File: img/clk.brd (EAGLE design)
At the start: 59.4 x 51.4 mm, 27 parts, among them IC1 MEGA8-P, IC2 DS1307, J1 22-27-2021-02

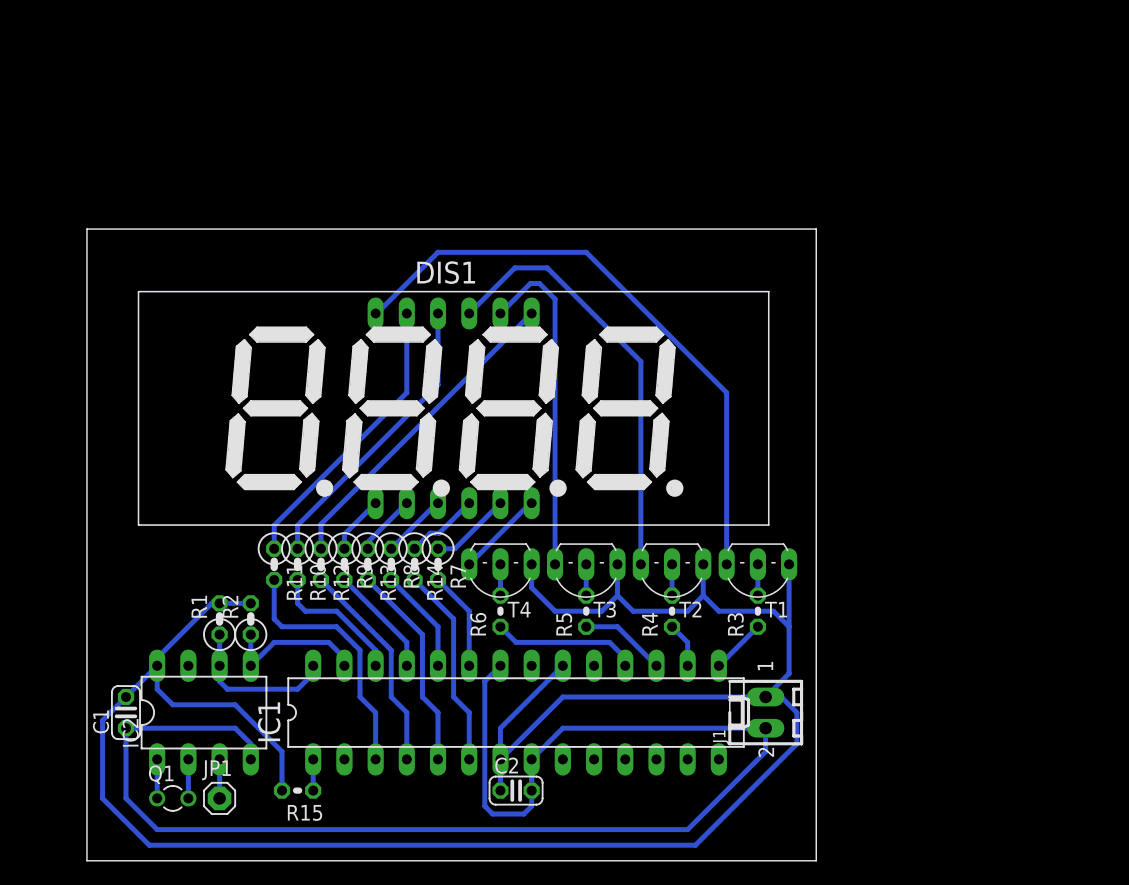
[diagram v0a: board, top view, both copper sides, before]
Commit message: Finished and tested version 2
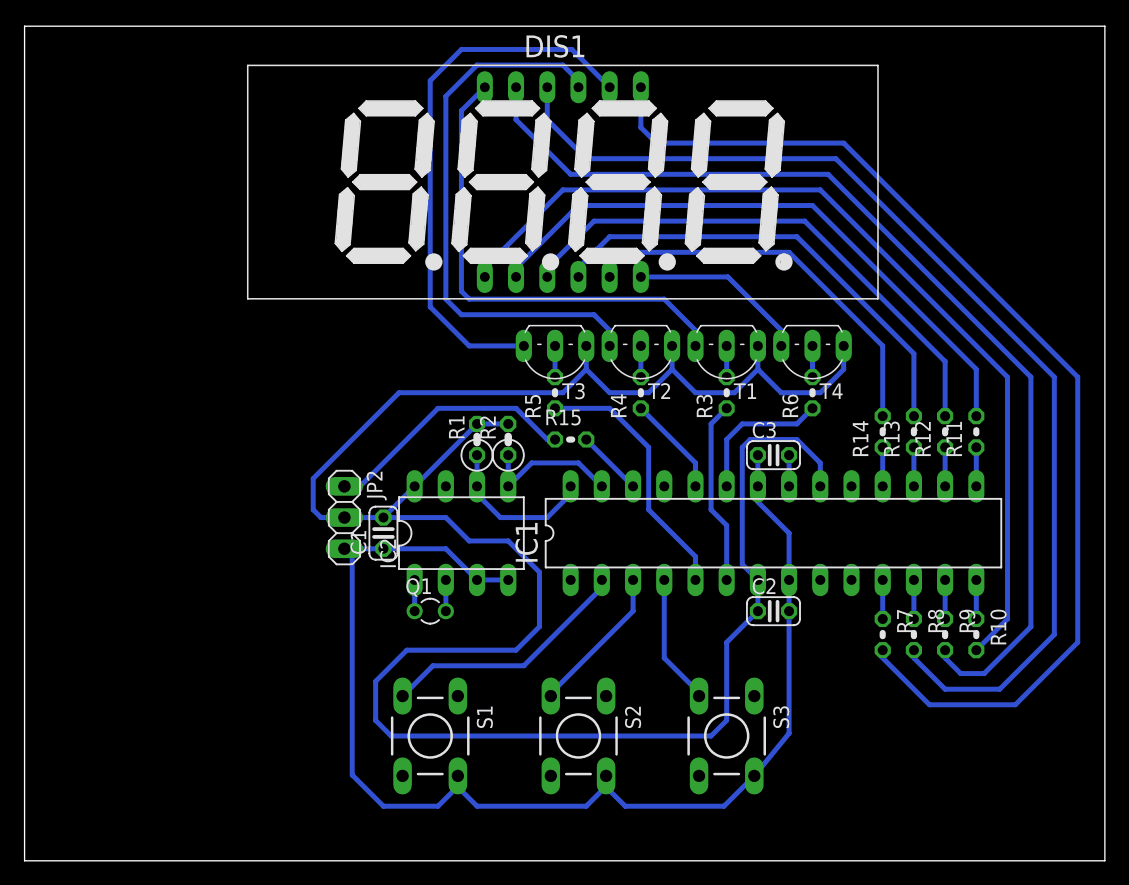
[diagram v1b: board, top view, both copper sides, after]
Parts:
- removed J1: 22-27-2021-02, con-molex:6410-02
- removed JP1: (no value), adafruit:1X01
- added C3: (no value), rcl:C025-024X044
- added JP2: (no value), pinhead:1X03
- added S1, S2, S3: DTS-6, switch-tact:DTS-6
- R10, R11, R12, R13, R14, R7, R8, R9: device rcl:0207/2V -> rcl:0204V
- moved R11 58.2 mm to (77.5, 34.9), turned to 90 degrees
- moved R10 55.5 mm to (77.5, 18.4)
- moved R12 51.9 mm to (74.9, 34.9), turned to 90 degrees
- moved R9 49.2 mm to (74.9, 18.4)
- moved R13 45.7 mm to (72.4, 34.9), turned to 90 degrees
- moved R8 42.9 mm to (72.4, 18.4)
- moved R14 39.6 mm to (69.8, 34.9), turned to 90 degrees
- moved R7 36.6 mm to (69.8, 18.4)
- moved R15 36.2 mm to (44.5, 34.3), turned to 0 degrees
- moved R6 31.0 mm to (64.1, 38.1)
- moved T4 31.0 mm to (64.1, 40.6)
- moved Q1 25.9 mm to (33.0, 20.3)
- moved IC2 25.5 mm to (35.6, 26.7)
- moved C1 25.5 mm to (29.2, 26.7)
- moved C2 25.5 mm to (61.0, 20.3)
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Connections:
- removed net N$13: IC1.1, R15.1
- new net BUTTON_1: IC1.2, S1.3, S1.4
- new net BUTTON_2: IC1.3, S2.3, S2.4
- new net BUTTON_3: IC1.4, S3.3, S3.4
- new net N$24: IC1.18, R14.1
- new net N$25: IC1.26, R15.2
- net +5V: now also JP2.2; no longer J1.1, R15.2
- net A: now also R9.2; no longer R11.1
- net B: now also R7.2; no longer R12.1
- net C: now also R13.2; no longer R14.1
- net D: now also R11.2; no longer R13.1
- net DP: now also R12.2; no longer R8.1
- net E: now also R10.2; no longer R9.1
- net F: now also R8.2; no longer R10.1
- net G: now also R14.2; no longer R7.1
- net GND: now also C3.1, IC2.3, JP2.3, S1.1, S1.2, S2.1, S2.2, S3.1, S3.2; no longer J1.2
- net N$14: now also IC1.24; no longer IC1.16
- net N$15: now also IC1.5; no longer IC1.17
- net N$16: now also IC1.11, R7.1; no longer IC1.18, R6.1
- net N$17: now also IC1.12, R8.1; no longer IC1.26, R10.2
- net N$18: now also IC1.13, R9.1; no longer IC1.3, R11.2
- net N$19: now also IC1.14, R10.1; no longer IC1.4, R12.2
- net N$20: now also IC1.15, R11.1; no longer IC1.5, R13.2
- net N$21: now also IC1.16, R12.1; no longer IC1.6, R14.2
- net N$22: now also IC1.17, R13.1; no longer IC1.15, R3.1
- net N$3: now also C3.2, IC1.21; no longer IC1.23, R7.2
- net N$4: now also JP2.1, R15.1; no longer IC1.24, R8.2
- net N$7: now also IC1.23, R6.1; no longer IC2.3, JP1.1
- net N$8: now also IC1.6, R3.1; no longer IC1.25, R9.2
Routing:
- net E: track 4.76 -> 75.5 mm
- net F: track 23.9 -> 88.5 mm
- net B: track 26.3 -> 89.0 mm
- net A: track 23.6 -> 83.3 mm
- net D: track 5.03 -> 49.6 mm
- net DP: track 5.35 -> 43.9 mm
- net C: track 5.98 -> 38.1 mm
- net G: track 6.62 -> 32.4 mm
- net BUTTON_1: track 0.00 -> 20.5 mm
- net N$18: track 20.6 -> 3.18 mm
- net D3: track 27.6 -> 44.3 mm
- net GND: track 118.1 -> 102.2 mm
- net N$19: track 17.5 -> 3.18 mm
- net N$15: track 7.03 -> 21.3 mm
- net N$20: track 17.0 -> 3.18 mm
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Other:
- board size 59.4 x 51.4 mm -> 87.9 x 67.9 mm
